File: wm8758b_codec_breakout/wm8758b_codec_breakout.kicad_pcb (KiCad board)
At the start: 2 copper layers, 40 x 40 mm, 21 parts, among them J1 Conn_01x12, J101 AudioJack3, J102 AudioJack3, J2 Conn_01x12, U1 WM8758B

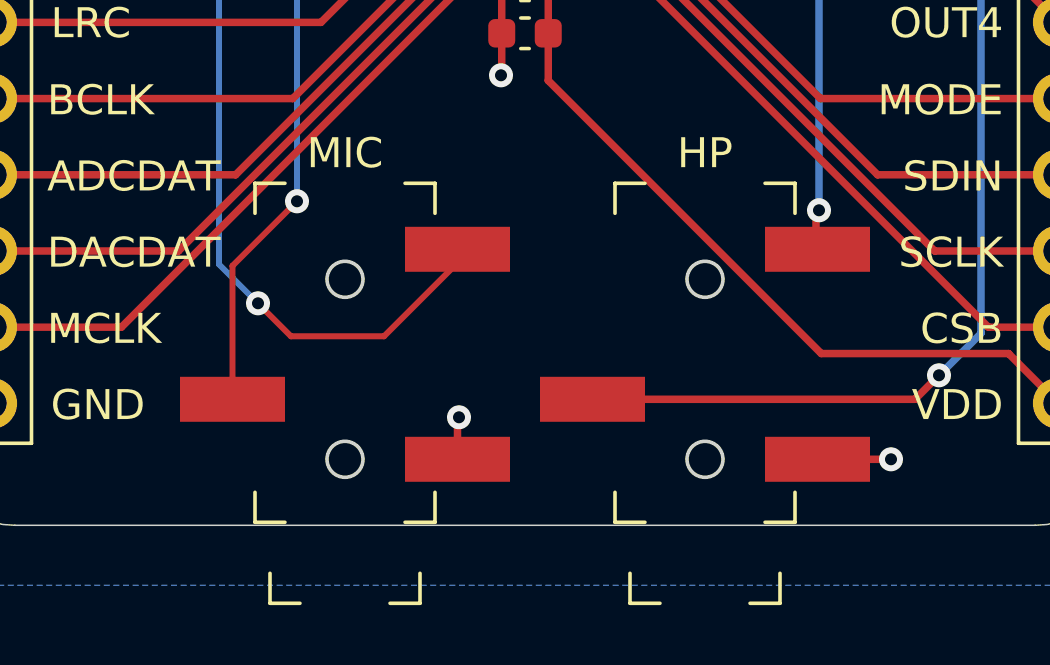
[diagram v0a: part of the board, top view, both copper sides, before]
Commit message: Order JLCPC V1
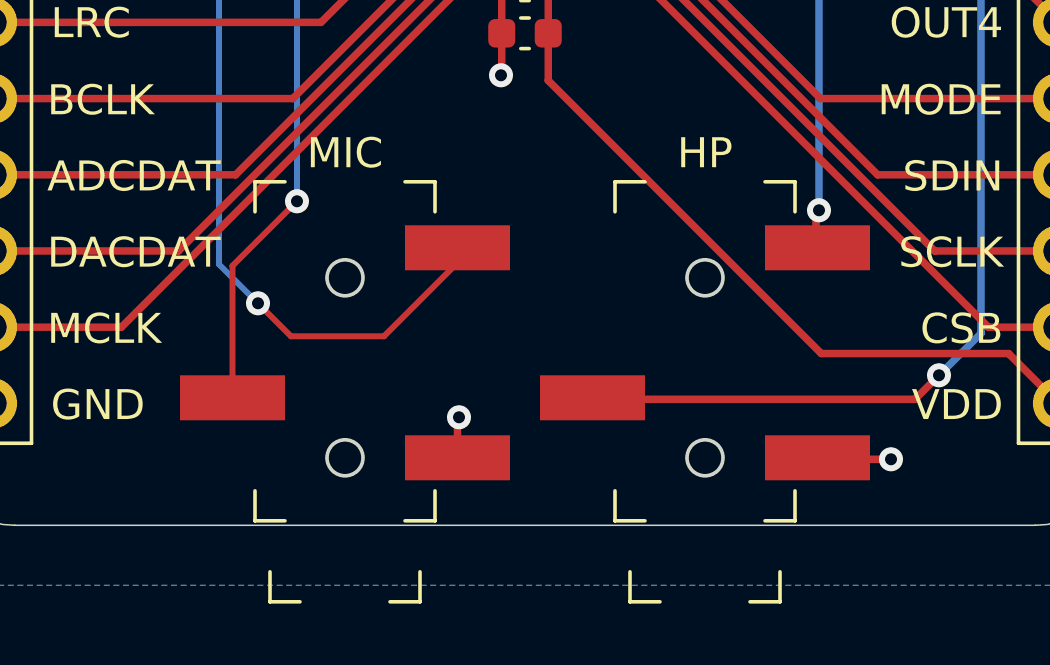
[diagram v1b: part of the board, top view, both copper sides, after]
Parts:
- moved J101 5.70 mm to (144.0, 94.2), turned to 90 degrees
- moved J102 5.70 mm to (156.0, 94.2), turned to 90 degrees
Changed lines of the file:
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@@
   )
   (footprint "WM8758B_breakout:PJ-320B-3A" (layer "F.Cu")
-    (at 144 99.9)
+    (at 144 94.2 90)
     (property "MSCS Part" "C707224")
     (property "Sheetfile" "wm8758b_codec_breakout.kicad_sch")
     (property "Sheetname" "")
     (attr smd)
-    (fp_text reference "J101" (at 0.15 -12.3 unlocked) (layer "F.Fab")
+    (fp_text reference "J101" (at 0.15 -12.3 90 unlocked) (layer "F.Fab")
       (effects (font (size 1 1) (thickness 0.15)))
     )
-    (fp_text value "AudioJack3" (at 0 4.1 unlocked) (layer "F.Fab")
+    (fp_text value "AudioJack3" (at 0 4.1 90 unlocked) (layer "F.Fab")
       (effects (font (size 1 1) (thickness 0.15)))
     )
-    (fp_text user "${REFERENCE}" (at 0 6 unlocked) (layer "F.Fab")
+    (fp_text user "${REFERENCE}" (at 0 6 90 unlocked) (layer "F.Fab")
       (effects (font (size 1 1) (thickness 0.15)))
     )
-    (fp_line (start -2.5 1.7) (end -2.5 2.7) (layer "F.SilkS") (width 0.12))
-    (fp_line (start 2 -11.3) (end 3 -11.3) (layer "F.SilkS") (width 0.12))
-    (fp_line (start -3 -10.3) (end -3 -11.3) (layer "F.SilkS") (width 0.12))
-    (fp_line (start 2.5 1.7) (end 2.5 2.7) (layer "F.SilkS") (width 0.12))
-    (fp_line (start -2.5 2.7) (end -1.5 2.7) (layer "F.SilkS") (width 0.12))
-    (fp_line (start -3 0) (end -2 0) (layer "F.SilkS") (width 0.12))
-    (fp_line (start 3 -1) (end 3 0) (layer "F.SilkS") (width 0.12))
-    (fp_line (start 3 -11.3) (end 3 -10.3) (layer "F.SilkS") (width 0.12))
-    (fp_line (start -3 -11.3) (end -2 -11.3) (layer "F.SilkS") (width 0.12))
-    (fp_line (start 2.5 2.7) (end 1.5 2.7) (layer "F.SilkS") (width 0.12))
-    (fp_line (start -3 -1) (end -3 0) (layer "F.SilkS") (width 0.12))
-    (fp_line (start 3 0) (end 2 0) (layer "F.SilkS") (width 0.12))
-    (fp_circle (center 0 -8.1) (end 0.6 -8.1) (layer "Edge.Cuts") (width 0.12) (fill none))
-    (fp_circle (center 0 -2.1) (end 0.6 -2.1) (layer "Edge.Cuts") (width 0.12) (fill none))
-    (fp_rect (start -5.6 -11.5) (end 5.6 2.9) (layer "F.CrtYd") (width 0.05) (fill none))
-    (fp_rect (start -3 0) (end 3 -11.3) (layer "F.Fab") (width 0.1) (fill none))
-    (fp_rect (start -2.5 0) (end 2.5 2.7) (layer "F.Fab") (width 0.1) (fill none))
-    (pad "R" smd rect (at -3.75 -4.1) (size 3.5 1.5) (layers "F.Cu" "F.Paste" "F.Mask")
+    (fp_line (start -8.35 -2.5) (end -8.35 -1.5) (layer "F.SilkS") (width 0.12))
+    (fp_line (start 5.65 -3) (end 5.65 -2) (layer "F.SilkS") (width 0.12))
+    (fp_line (start -7.35 -2.5) (end -8.35 -2.5) (layer "F.SilkS") (width 0.12))
+    (fp_line (start -5.65 3) (end -5.65 2) (layer "F.SilkS") (width 0.12))
+    (fp_line (start -4.65 -3) (end -5.65 -3) (layer "F.SilkS") (width 0.12))
+    (fp_line (start 5.65 2) (end 5.65 3) (layer "F.SilkS") (width 0.12))
+    (fp_line (start -8.35 2.5) (end -8.35 1.5) (layer "F.SilkS") (width 0.12))
+    (fp_line (start -4.65 3) (end -5.65 3) (layer "F.SilkS") (width 0.12))
+    (fp_line (start -7.35 2.5) (end -8.35 2.5) (layer "F.SilkS") (width 0.12))
+    (fp_line (start -5.65 -3) (end -5.65 -2) (layer "F.SilkS") (width 0.12))
+    (fp_line (start 5.65 3) (end 4.65 3) (layer "F.SilkS") (width 0.12))
+    (fp_line (start 4.65 -3) (end 5.65 -3) (layer "F.SilkS") (width 0.12))
+    (fp_circle (center -3.55 0) (end -3.55 0.6) (layer "Edge.Cuts") (width 0.12) (fill none))
+    (fp_circle (center 2.45 0) (end 2.45 0.6) (layer "Edge.Cuts") (width 0.12) (fill none))
+    (fp_rect (start 5.85 -5.6) (end -8.55 5.6) (layer "F.CrtYd") (width 0.05) (fill none))
+    (fp_rect (start -5.65 -2.5) (end -8.35 2.5) (layer "F.Fab") (width 0.1) (fill none))
+    (fp_rect (start -5.65 -3) (end 5.65 3) (layer "F.Fab") (width 0.1) (fill none))
+    (pad "R" smd rect (at -1.55 -3.75) (size 3.5 1.5) (layers "F.Cu" "F.Paste" "F.Mask")
       (net 12 "RIN") (pintype "passive"))
-    (pad "S" smd rect (at 3.75 -2.1) (size 3.5 1.5) (layers "F.Cu" "F.Paste" "F.Mask")
+    (pad "S" smd rect (at -3.55 3.75) (size 3.5 1.5) (layers "F.Cu" "F.Paste" "F.Mask")
       (net 1 "GND") (pintype "passive"))
-    (pad "T" smd rect (at 3.75 -9.1) (size 3.5 1.5) (layers "F.Cu" "F.Paste" "F.Mask")
+    (pad "T" smd rect (at 3.45 3.75) (size 3.5 1.5) (layers "F.Cu" "F.Paste" "F.Mask")
       (net 14 "LIN") (pintype "passive"))
   )
@@
   )
   (footprint "WM8758B_breakout:PJ-320B-3A" (layer "F.Cu")
-    (at 156 99.9)
+    (at 156 94.2 90)
     (property "MSCS Part" "C707224")
     (property "Sheetfile" "wm8758b_codec_breakout.kicad_sch")
     (property "Sheetname" "")
     (attr smd)
-    (fp_text reference "J102" (at 0.15 -12.3 unlocked) (layer "F.Fab")
+    (fp_text reference "J102" (at 0.15 -12.3 90 unlocked) (layer "F.Fab")
       (effects (font (size 1 1) (thickness 0.15)))
     )
-    (fp_text value "AudioJack3" (at 0 4.1 unlocked) (layer "F.Fab")
+    (fp_text value "AudioJack3" (at 0 4.1 90 unlocked) (layer "F.Fab")
       (effects (font (size 1 1) (thickness 0.15)))
     )
-    (fp_text user "${REFERENCE}" (at 0 6 unlocked) (layer "F.Fab")
+    (fp_text user "${REFERENCE}" (at 0 6 90 unlocked) (layer "F.Fab")
       (effects (font (size 1 1) (thickness 0.15)))
     )
-    (fp_line (start 2.5 2.7) (end 1.5 2.7) (layer "F.SilkS") (width 0.12))
-    (fp_line (start -3 -10.3) (end -3 -11.3) (layer "F.SilkS") (width 0.12))
-    (fp_line (start 3 -11.3) (end 3 -10.3) (layer "F.SilkS") (width 0.12))
-    (fp_line (start 2 -11.3) (end 3 -11.3) (layer "F.SilkS") (width 0.12))
-    (fp_line (start 3 0) (end 2 0) (layer "F.SilkS") (width 0.12))
-    (fp_line (start -2.5 1.7) (end -2.5 2.7) (layer "F.SilkS") (width 0.12))
-    (fp_line (start -3 -1) (end -3 0) (layer "F.SilkS") (width 0.12))
-    (fp_line (start 3 -1) (end 3 0) (layer "F.SilkS") (width 0.12))
-    (fp_line (start -2.5 2.7) (end -1.5 2.7) (layer "F.SilkS") (width 0.12))
-    (fp_line (start 2.5 1.7) (end 2.5 2.7) (layer "F.SilkS") (width 0.12))
-    (fp_line (start -3 0) (end -2 0) (layer "F.SilkS") (width 0.12))
-    (fp_line (start -3 -11.3) (end -2 -11.3) (layer "F.SilkS") (width 0.12))
-    (fp_circle (center 0 -2.1) (end 0.6 -2.1) (layer "Edge.Cuts") (width 0.12) (fill none))
-    (fp_circle (center 0 -8.1) (end 0.6 -8.1) (layer "Edge.Cuts") (width 0.12) (fill none))
-    (fp_rect (start -5.6 -11.5) (end 5.6 2.9) (layer "F.CrtYd") (width 0.05) (fill none))
-    (fp_rect (start -3 0) (end 3 -11.3) (layer "F.Fab") (width 0.1) (fill none))
-    (fp_rect (start -2.5 0) (end 2.5 2.7) (layer "F.Fab") (width 0.1) (fill none))
-    (pad "R" smd rect (at -3.75 -4.1) (size 3.5 1.5) (layers "F.Cu" "F.Paste" "F.Mask")
+    (fp_line (start -7.35 -2.5) (end -8.35 -2.5) (layer "F.SilkS") (width 0.12))
+    (fp_line (start -7.35 2.5) (end -8.35 2.5) (layer "F.SilkS") (width 0.12))
+    (fp_line (start 5.65 3) (end 4.65 3) (layer "F.SilkS") (width 0.12))
+    (fp_line (start -4.65 -3) (end -5.65 -3) (layer "F.SilkS") (width 0.12))
+    (fp_line (start -8.35 2.5) (end -8.35 1.5) (layer "F.SilkS") (width 0.12))
+    (fp_line (start -5.65 -3) (end -5.65 -2) (layer "F.SilkS") (width 0.12))
+    (fp_line (start -8.35 -2.5) (end -8.35 -1.5) (layer "F.SilkS") (width 0.12))
+    (fp_line (start -4.65 3) (end -5.65 3) (layer "F.SilkS") (width 0.12))
+    (fp_line (start 5.65 -3) (end 5.65 -2) (layer "F.SilkS") (width 0.12))
+    (fp_line (start 4.65 -3) (end 5.65 -3) (layer "F.SilkS") (width 0.12))
+    (fp_line (start -5.65 3) (end -5.65 2) (layer "F.SilkS") (width 0.12))
+    (fp_line (start 5.65 2) (end 5.65 3) (layer "F.SilkS") (width 0.12))
+    (fp_circle (center 2.45 0) (end 2.45 0.6) (layer "Edge.Cuts") (width 0.12) (fill none))
+    (fp_circle (center -3.55 0) (end -3.55 0.6) (layer "Edge.Cuts") (width 0.12) (fill none))
+    (fp_rect (start 5.85 -5.6) (end -8.55 5.6) (layer "F.CrtYd") (width 0.05) (fill none))
+    (fp_rect (start -5.65 -3) (end 5.65 3) (layer "F.Fab") (width 0.1) (fill none))
+    (fp_rect (start -5.65 -2.5) (end -8.35 2.5) (layer "F.Fab") (width 0.1) (fill none))
+    (pad "R" smd rect (at -1.55 -3.75) (size 3.5 1.5) (layers "F.Cu" "F.Paste" "F.Mask")
       (net 17 "ROUT1") (pintype "passive"))
-    (pad "S" smd rect (at 3.75 -2.1) (size 3.5 1.5) (layers "F.Cu" "F.Paste" "F.Mask")
+    (pad "S" smd rect (at -3.55 3.75) (size 3.5 1.5) (layers "F.Cu" "F.Paste" "F.Mask")
       (net 1 "GND") (pintype "passive"))
-    (pad "T" smd rect (at 3.75 -9.1) (size 3.5 1.5) (layers "F.Cu" "F.Paste" "F.Mask")
+    (pad "T" smd rect (at 3.45 3.75) (size 3.5 1.5) (layers "F.Cu" "F.Paste" "F.Mask")
       (net 16 "LOUT1") (pintype "passive"))
   )
